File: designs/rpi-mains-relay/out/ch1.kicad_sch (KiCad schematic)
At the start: 8 parts, among them J2 2606-3102/020-000, K1 G5RL-1A-E-TV8 DC5, Q1 AO3400A

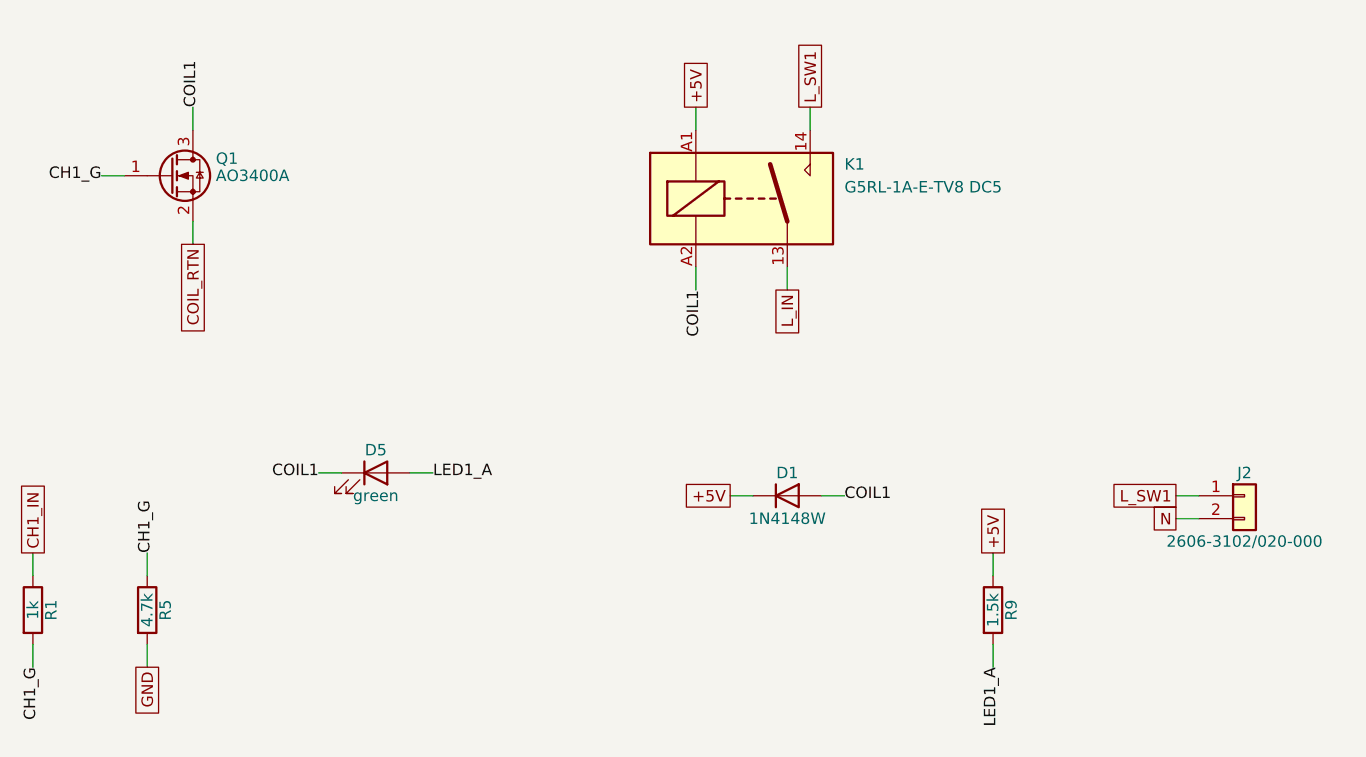
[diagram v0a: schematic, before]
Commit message: designs: work-in-progress (Prius encoding and relay-board rework under way)
Co-Authored-By: Claude Opus 5.5 <noreply@anthropic.com>
Claude-Session: https://claude.ai/code/session_01VFJn9VbX8h27kf4LpLwEtn
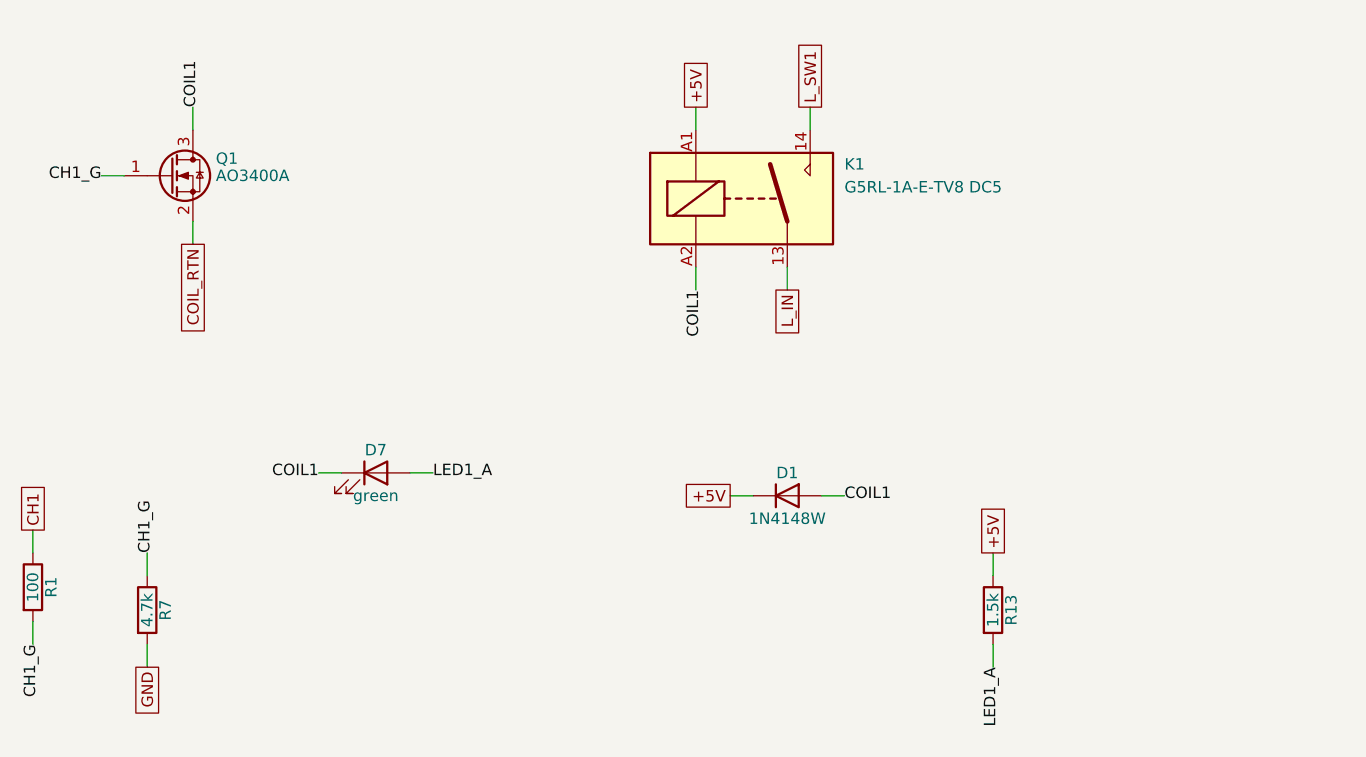
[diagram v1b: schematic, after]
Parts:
- removed D5: green, LED_SMD:LED_0603_1608Metric, symbol Device:LED
- removed J2: 2606-3102/020-000, custom:WAGO_2606-3102_020-000, symbol Connector_Generic:Conn_01x02
- removed R5: 4.7k, Resistor_SMD:R_0603_1608Metric, symbol Device:R
- removed R9: 1.5k, Resistor_SMD:R_0603_1608Metric, symbol Device:R
- added D7: green, LED_SMD:LED_0603_1608Metric, symbol Device:LED
- added R13: 1.5k, Resistor_SMD:R_0603_1608Metric, symbol Device:R
- added R7: 4.7k, Resistor_SMD:R_0603_1608Metric, symbol Device:R
- R1: value 1k -> 100; MPN RC0603FR-071KL -> RC0603FR-07100RL
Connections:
- net +5V: now also R13.1
- net CH1_G: now also R7.1
- net COIL1: now also D7.1 (K)
- net GND: now also R7.2
- net LED1_A: now also D7.2 (A), R13.2
- net CH1_IN renamed CH1
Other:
- title: Channel 1: relay K1, driver Q1, output J2 -> Outlet 1: relay K1, driver Q1
- moved on the sheet: R1
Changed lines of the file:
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@@
 	(paper "A4")
 	(title_block
-		(title "Channel 1: relay K1, driver Q1, output J2")
+		(title "Outlet 1: relay K1, driver Q1")
 		(date "2026-10-23")
 		(rev "A")
 		(company "kaesynth")
-		(comment 1 "CH1_IN = Pi pin 11 (BCM17); K1 switches L_IN to L_SW1; J2 = OUT1 L/N")
-		(comment 2 "RPi 4-channel 120 VAC relay board (4-11/16 in box) — generated by kaesynth from design.py; do not edit by hand")
+		(comment 1 "CH1 = Pi pin 11 (BCM17); K1 switches L_IN to L_SW1 -> J2.1")
+		(comment 2 "RPi Zero 2 W six-outlet 120 VAC relay board (polycarbonate enclosure) — generated by kaesynth from design.py; do not edit by hand")
 	)
 	(symbol
 		(lib_id "Device:R")
-		(at 27.94 96.52 0)
+		(at 27.94 93.98 0)
 		(unit 1)
 		(exclude_from_sim no)
@@
 		(dnp no)
 		(property "Reference" "R1"
-			(at 29.972 96.52 90)
-			(effects
-				(font (size 1.27 1.27))
-			)
-		)
-		(property "Value" "1k"
-			(at 27.94 96.52 90)
+			(at 29.972 93.98 90)
+			(effects
+				(font (size 1.27 1.27))
+			)
+		)
+		(property "Value" "100"
+			(at 27.94 93.98 90)
 			(effects
 				(font (size 1.27 1.27))
@@
 		)
 		(property "Footprint" "Resistor_SMD:R_0603_1608Metric"
-			(at 27.94 96.52 0)
+			(at 27.94 93.98 0)
 			(hide yes)
 			(effects
@@
 		)
 		(property "Datasheet" "https://yageogroup.com/content/datasheet/asset/file/PYU-RC_GROUP_51_ROHS_L"
-			(at 27.94 96.52 0)
-			(hide yes)
-			(effects
-				(font (size 1.27 1.27))
-			)
-		)
-		(property "Description" "Resistor 1k 1% 0603"
-			(at 27.94 96.52 0)
-			(hide yes)
-			(effects
-				(font (size 1.27 1.27))
-			)
-		)
-		(property "MPN" "RC0603FR-071KL"
-			(at 27.94 96.52 0)
+			(at 27.94 93.98 0)
+			(hide yes)
+			(effects
+				(font (size 1.27 1.27))
+			)
+		)
+		(property "Description" "Resistor 100 1% 0603"
+			(at 27.94 93.98 0)
+			(hide yes)
+			(effects
+				(font (size 1.27 1.27))
+			)
+		)
+		(property "MPN" "RC0603FR-07100RL"
+			(at 27.94 93.98 0)
 			(hide yes)
 			(effects
@@
 		)
 		(property "Manufacturer" "YAGEO"
-			(at 27.94 96.52 0)
+			(at 27.94 93.98 0)
 			(hide yes)
 			(effects
@@
 		)
 		(property "Block" "ch1"
-			(at 27.94 96.52 0)
+			(at 27.94 93.98 0)
 			(hide yes)
 			(effects
@@
 		)
 		(property "Component Class" "ch1"
-			(at 27.94 96.52 0)
+			(at 27.94 93.98 0)
 			(hide yes)
 			(effects
@@
 		)
 		(property "Tolerance" "1%"
-			(at 27.94 96.52 0)
+			(at 27.94 93.98 0)
 			(hide yes)
 			(effects
@@
 		)
 		(property "Package" "0603"
-			(at 27.94 96.52 0)
+			(at 27.94 93.98 0)
 			(hide yes)
 			(effects
@@
 	)
 	(wire
-		(pts (xy 27.94 92.71) (xy 27.94 90.17))
-		(stroke
-			(width 0)
-			(type default)
-		)
-	)
-	(global_label "CH1_IN"
+		(pts (xy 27.94 90.17) (xy 27.94 87.63))
+		(stroke
+			(width 0)
+			(type default)
+		)
+	)
+	(global_label "CH1"
 		(shape passive)
-		(at 27.94 90.17 90)
+		(at 27.94 87.63 90)
 		(fields_autoplaced yes)
 		(effects
@@
 		)
 		(property "Intersheetrefs" "${INTERSHEET_REFS}"
-			(at 27.94 90.17 0)
-			(hide yes)
-			(effects
-				(font (size 1.27 1.27))
-			)
-		)
-	)
-	(wire
-		(pts (xy 27.94 100.33) (xy 27.94 102.87))
+			(at 27.94 87.63 0)
+			(hide yes)
+			(effects
+				(font (size 1.27 1.27))
+			)
+		)
+	)
+	(wire
+		(pts (xy 27.94 97.79) (xy 27.94 100.33))
 		(stroke
 			(width 0)
@@
 	)
 	(label "CH1_G"
-		(at 27.94 102.87 270)
+		(at 27.94 100.33 270)
 		(fields_autoplaced yes)
 		(effects
@@
 		(on_board yes)
 		(dnp no)
-		(property "Reference" "R5"
+		(property "Reference" "R7"
 			(at 42.672 96.52 90)
 			(effects
@@
 			(project "rpi-mains-relay"
 				(path "/a30cabb5-b934-5e97-9aeb-aaefec3ba07a/d5d3af06-bb94-5568-b155-db1df6270ff3"
-					(reference "R5")
+					(reference "R7")
 					(unit 1)
 				)
@@
 		(on_board yes)
 		(dnp no)
-		(property "Reference" "D5"
+		(property "Reference" "D7"
 			(at 66.04 78.74 0)
 			(effects
@@
 			(project "rpi-mains-relay"
 				(path "/a30cabb5-b934-5e97-9aeb-aaefec3ba07a/d5d3af06-bb94-5568-b155-db1df6270ff3"
-					(reference "D5")
+					(reference "D7")
 					(unit 1)
 				)
@@
 		(on_board yes)
 		(dnp no)
-		(property "Reference" "R9"
+		(property "Reference" "R13"
 			(at 136.652 96.52 90)
 			(effects
@@
 			(project "rpi-mains-relay"
 				(path "/a30cabb5-b934-5e97-9aeb-aaefec3ba07a/d5d3af06-bb94-5568-b155-db1df6270ff3"
-					(reference "R9")
+					(reference "R13")
 					(unit 1)
 				)
@@
 		)
 	)
-	(symbol
-		(lib_id "Connector_Generic:Conn_01x02")
-		(at 162.56 83.82 0)
-		(unit 1)
-		(exclude_from_sim no)
-		(in_bom yes)
-		(on_board yes)
-		(dnp no)
-		(property "Reference" "J2"
-			(at 162.56 81.28 0)
-			(effects
-				(font (size 1.27 1.27))
-			)
-		)
-		(property "Value" "2606-3102/020-000"
-			(at 162.56 88.9 0)
-			(effects
-				(font (size 1.27 1.27))
-			)
-		)
-		(property "Footprint" "custom:WAGO_2606-3102_020-000"
-			(at 162.56 83.82 0)
-			(hide yes)
-			(effects
-				(font (size 1.27 1.27))
-			)
-		)
-		(property "Datasheet" "https://www.wago.com/2606-3102/020-000"
-			(at 162.56 83.82 0)
-			(hide yes)
-			(effects
-				(font (size 1.27 1.27))
-			)
-		)
-		(property "Description" "PCB terminal block 2-pole, lever, push-in CAGE CLAMP, 6 mm2, 7.5 mm pitch, staggered pins"
-			(at 162.56 83.82 0)
-			(hide yes)
-			(effects
-				(font (size 1.27 1.27))
-			)
-		)
-		(property "MPN" "2606-3102/020-000"
-			(at 162.56 83.82 0)
-			(hide yes)
-			(effects
-				(font (size 1.27 1.27))
-			)
-		)
-		(property "Manufacturer" "WAGO"
-			(at 162.56 83.82 0)
-			(hide yes)
-			(effects
-				(font (size 1.27 1.27))
-			)
-		)
-		(property "Block" "ch1"
-			(at 162.56 83.82 0)
-			(hide yes)
-			(effects
-				(font (size 1.27 1.27))
-			)
-		)
-		(property "Component Class" "ch1"
-			(at 162.56 83.82 0)
-			(hide yes)
-			(effects
-				(font (size 1.27 1.27))
-			)
-		)
-		(pin "1"
-		)
-		(pin "2"
-		)
-		(instances
-			(project "rpi-mains-relay"
-				(path "/a30cabb5-b934-5e97-9aeb-aaefec3ba07a/d5d3af06-bb94-5568-b155-db1df6270ff3"
-					(reference "J2")
-					(unit 1)
-				)
-			)
-		)
-	)
-	(wire
-		(pts (xy 157.48 83.82) (xy 154.94 83.82))
-		(stroke
-			(width 0)
-			(type default)
-		)
-	)
-	(global_label "L_SW1"
-		(shape passive)
-		(at 154.94 83.82 180)
-		(fields_autoplaced yes)
-		(effects
-			(font (size 1.27 1.27))
-			(justify right)
-		)
-		(property "Intersheetrefs" "${INTERSHEET_REFS}"
-			(at 154.94 83.82 0)
-			(hide yes)
-			(effects
-				(font (size 1.27 1.27))
-			)
-		)
-	)
-	(wire
-		(pts (xy 157.48 86.36) (xy 154.94 86.36))
-		(stroke
-			(width 0)
-			(type default)
-		)
-	)
-	(global_label "N"
-		(shape passive)
-		(at 154.94 86.36 180)
-		(fields_autoplaced yes)
-		(effects
-			(font (size 1.27 1.27))
-			(justify right)
-		)
-		(property "Intersheetrefs" "${INTERSHEET_REFS}"
-			(at 154.94 86.36 0)
-			(hide yes)
-			(effects
-				(font (size 1.27 1.27))
-			)
-		)
-	)
